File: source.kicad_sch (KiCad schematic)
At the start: 12 parts, among them T1 25, U3 LM78M05_TO220, U4 LM78M05_TO220

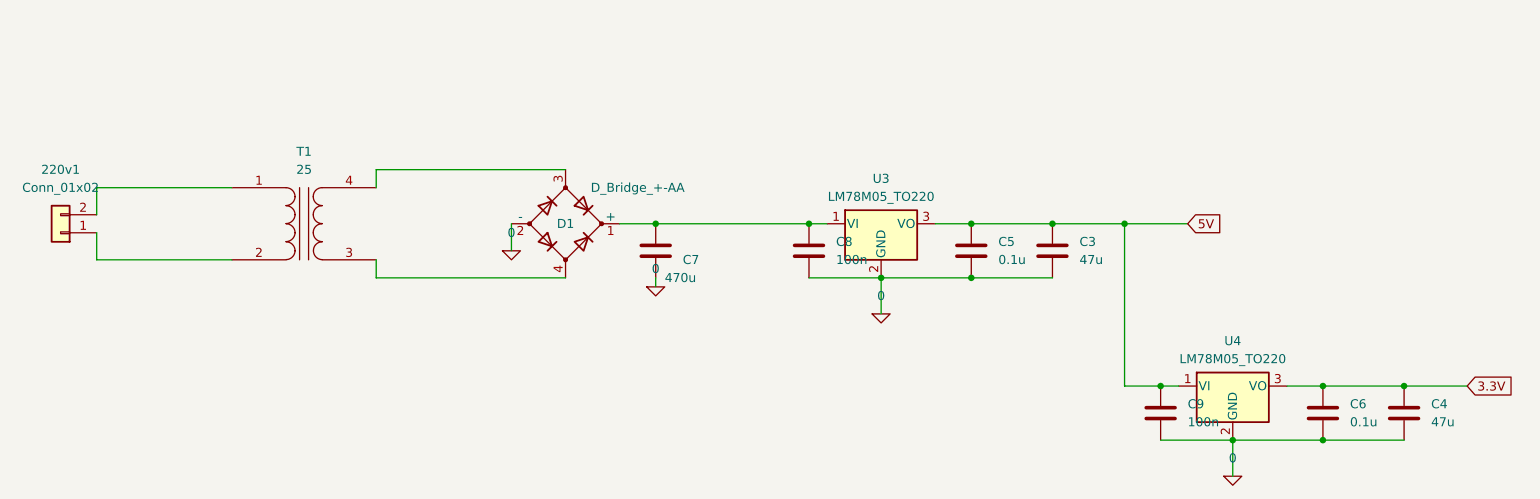
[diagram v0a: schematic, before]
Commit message: com
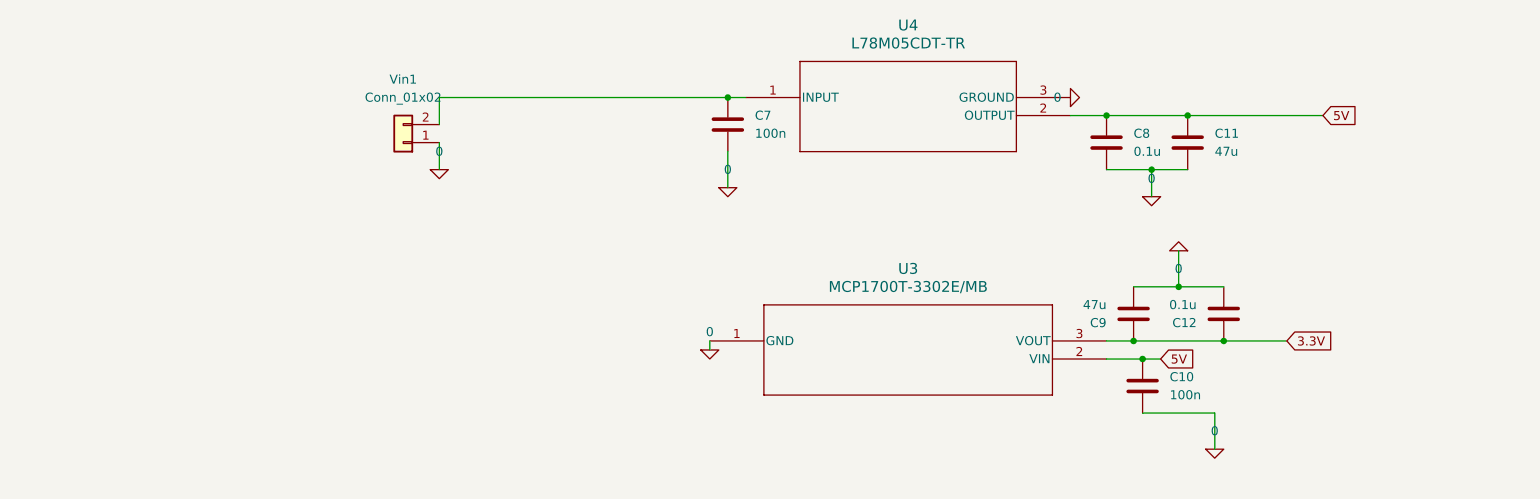
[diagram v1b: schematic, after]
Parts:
- removed C6: 0.1u, Capacitor_THT:CP_Radial_D8.0mm_P3.80mm, symbol Device:C
- removed C7: 470u, Capacitor_THT:CP_Radial_D8.0mm_P3.80mm, symbol Device:C
- removed C9: 100n, Capacitor_THT:CP_Radial_D8.0mm_P3.80mm, symbol Device:C
- removed D1: D_Bridge_+-AA, Connector_PinHeader_2.54mm:PinHeader_1x04_P2.54mm_Vertical, symbol Device:D_Bridge_+-AA
- removed T1: 25, Transformer_THT:Transformer_Toroid_Horizontal_D18.0mm, symbol Device:Transformer_1P_1S
- removed U3, U4: LM78M05_TO220, Package_TO_SOT_THT:TO-220-3_Vertical, symbol Regulator_Linear:LM78M05_TO220
- added C10: 100n, Capacitor_SMD:C_1210_3225Metric, symbol Device:C
- added C12: 0.1u, Capacitor_SMD:C_0805_2012Metric, symbol Device:C
- added U3: MCP1700T-3302E/MB, reg33:SOT-89_3MC_MCH, symbol 2023-12-18_18-15-44:MCP1700T-3302E_MB
- added U4: L78M05CDT-TR, reg5:DPAK_STM, symbol 2023-12-18_18-19-47:L78M05CDT-TR
- C7: renamed from C8; footprint Capacitor_THT:CP_Radial_D8.0mm_P3.80mm -> Capacitor_SMD:C_1210_3225Metric
- C8: renamed from C5; footprint Capacitor_THT:CP_Radial_D8.0mm_P3.80mm -> Capacitor_SMD:C_0805_2012Metric
- renumbered C3 to C11, C4 to C9, 220v1 to Vin1
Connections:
- net 0: now also Vin1.1 (Pin_1), C10.2, C12.2, U3.1 (GND), U4.3 (GROUND)
- net 3.3V: now also C12.1, U3.3 (VOUT)
- net 5V: now also C10.1, U3.2 (VIN), U4.2 (OUTPUT)
- net at C7.1: now also Vin1.2 (Pin_2), U4.1 (INPUT)
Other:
- moved on the sheet: C11, C7, C8, C9, Vin1
